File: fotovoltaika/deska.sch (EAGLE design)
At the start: 16 parts

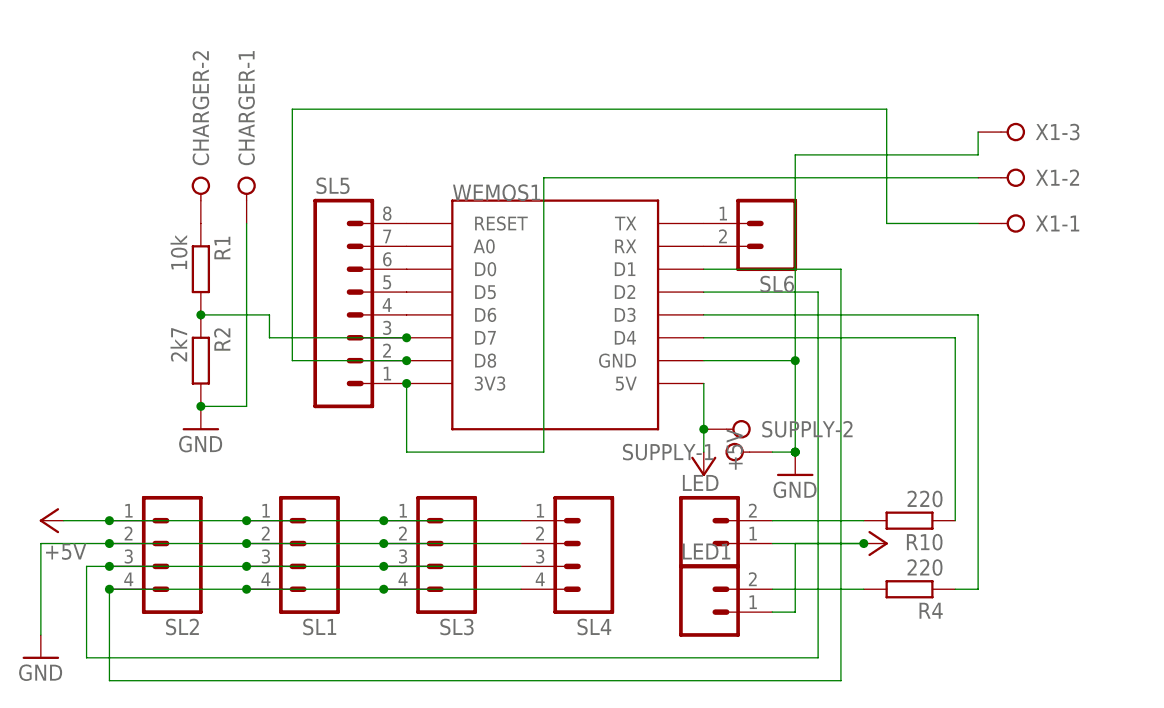
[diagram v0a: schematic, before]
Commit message: uprava desky
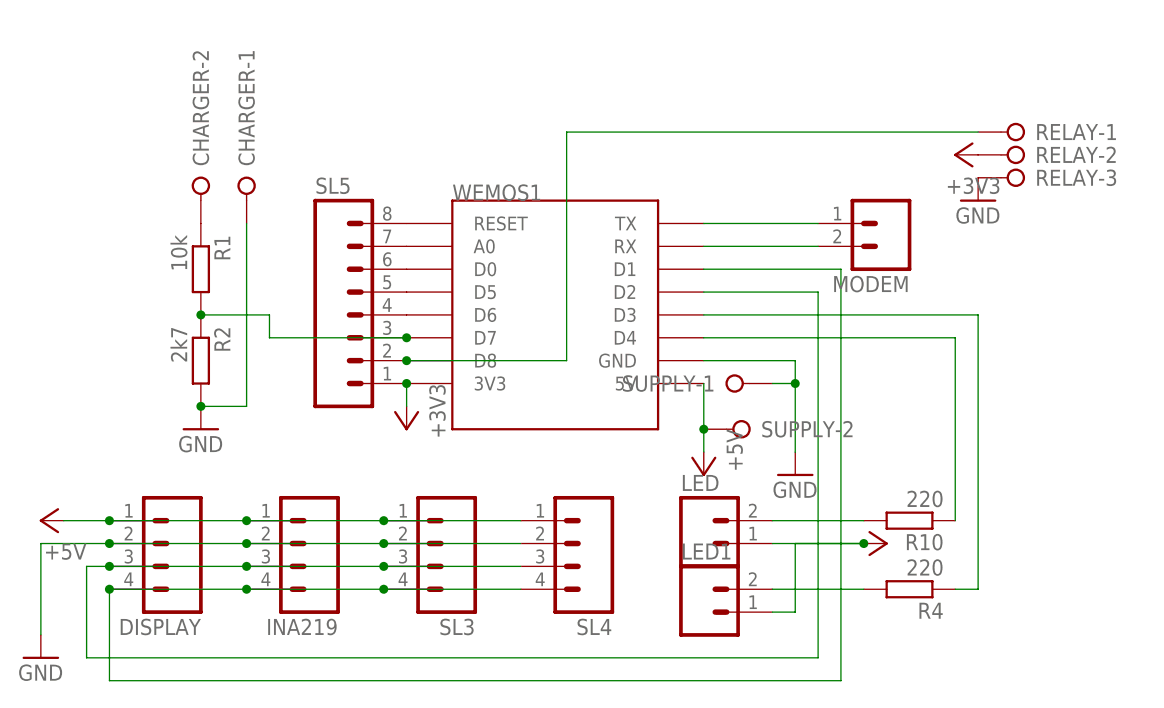
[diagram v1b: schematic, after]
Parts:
- removed SL6: (no value), con-amp-quick:M02
- removed X1: (no value), con-wago-508:W237-3E
- added MODEM: (no value), con-amp-quick:M02
- added RELAY: (no value), con-wago-508:W237-3E
- renumbered SL1 to INA219, SL2 to DISPLAY
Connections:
- removed net N$18: SL5.1, WEMOS1.3V3, X1-2.KL
- new net +3V3: RELAY-2.KL, SL5.1, WEMOS1.3V3
- net GND: now also RELAY-3.KL; no longer X1-3.KL
- net N$14: now also MODEM.1; no longer SL6.1
- net N$15: now also MODEM.2; no longer SL6.2
- net N$4: now also RELAY-1.KL; no longer X1-1.KL
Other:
- moved on the sheet: SUPPLY-1
